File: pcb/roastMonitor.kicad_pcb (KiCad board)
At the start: 2 copper layers, 45 x 60 mm, 73 parts, among them J1 USB_C_Receptacle_USB2.0_16P, J2 Conn_01x02, J3 Conn_01x02, J4 Conn_01x04, J5 Conn_01x04, U1 REF3040, U2 USBLC6-2SC6, U3 OPA2333xxD, U4 CH32X033F8P6, U5 MCP9701A, U6 OPA2333xxD

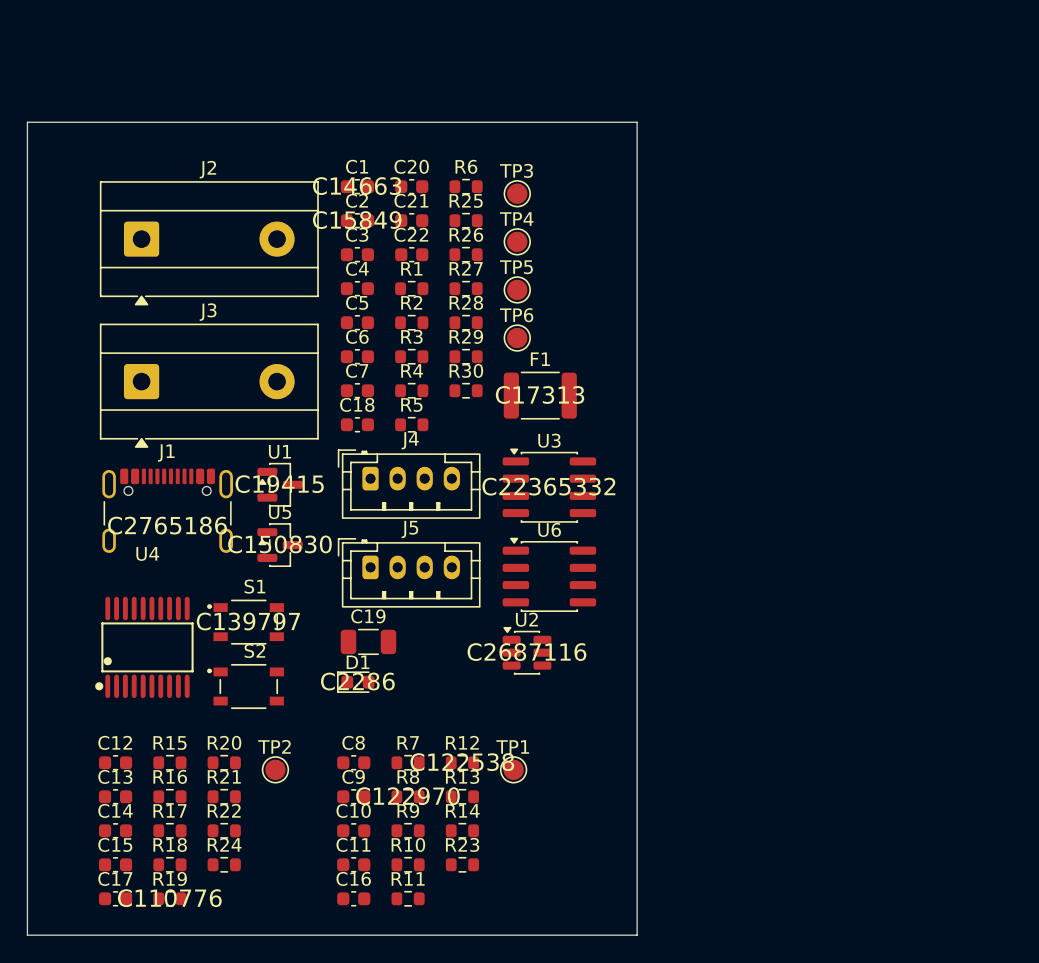
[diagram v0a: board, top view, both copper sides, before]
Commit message: Update PCB
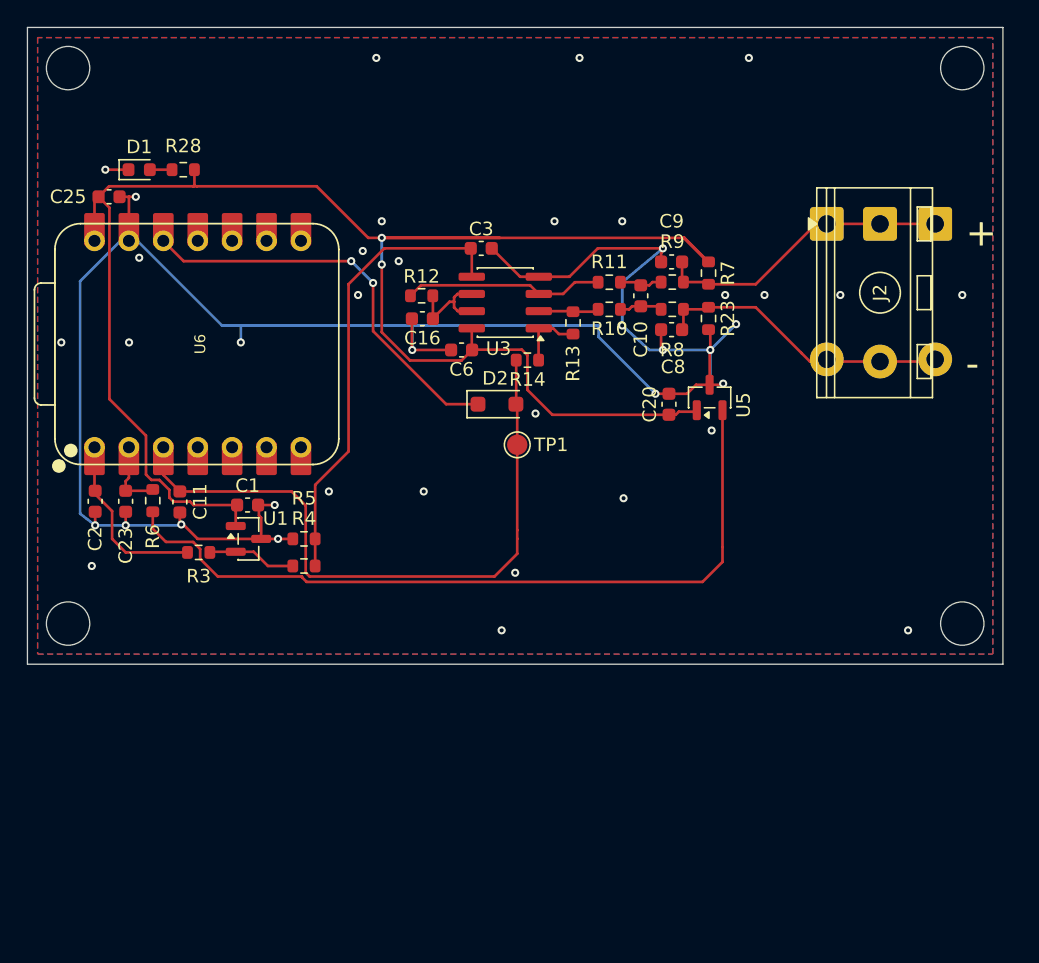
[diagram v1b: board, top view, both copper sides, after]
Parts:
- removed C12, C13, C14, C17, C18, C21, C22, C4, C5, C7: 100n, Capacitor_SMD:C_0603_1608Metric
- removed C15: 1u, Capacitor_SMD:C_0603_1608Metric
- removed C19: 4.7u, Capacitor_SMD:C_1206_3216Metric
- removed F1: Polyfuse, Fuse:Fuse_1812_4532Metric
- removed J1: USB_C_Receptacle_USB2.0_16P, Connector_USB:USB_C_Receptacle_GCT_USB4105-xx-A_16P_TopMnt_Horizontal
- removed J3: Conn_01x02, TerminalBlock_MetzConnect:TerminalBlock_MetzConnect_Type067_RT01902HDWC_1x02_P10.00mm_Horizontal
- removed J4, J5: Conn_01x04, Connector_JST:JST_PH_B4B-PH-K_1x04_P2.00mm_Vertical
- removed R1, R2: 5.1k, Resistor_SMD:R_0603_1608Metric
- removed R15: 10M, Resistor_SMD:R_0603_1608Metric
- removed R16, R17: 100±0.1%, Resistor_SMD:R_0603_1608Metric
- removed R18, R19: 1k±0.1%, Resistor_SMD:R_0603_1608Metric
- removed R20, R21: 100k±0.1%, Resistor_SMD:R_0603_1608Metric
- removed R22: 1k, Resistor_SMD:R_0603_1608Metric
- removed R24: 0, Resistor_SMD:R_0603_1608Metric
- removed R25, R26, R29, R30: 22, Resistor_SMD:R_0603_1608Metric
- removed R27: 10k, Resistor_SMD:R_0603_1608Metric
- removed S1, S2: SKRPACE010, private:SW_SKRPACE010
- removed TP2, TP3, TP4, TP5, TP6: TestPoint, TestPoint:TestPoint_Pad_D1.5mm
- removed U2: USBLC6-2SC6, Package_TO_SOT_SMD:SOT-23-6
- removed U4: CH32X033F8P6, private:TSSOP-20_L6.5-W4.4-P0.65-LS6.4-BL
- added ?: , , F.Cu at (197.0, 87.5)
- added ?: , , F.Cu at (189.0, 87.5)
- added ?: , , F.Cu at (189.0, 77.5)
- added ?: , , F.Cu at (197.0, 77.5)
- added C23: 1u, Capacitor_SMD:C_0603_1608Metric, F.Cu at (137.2, 98.0)
- added C25: 100n, Capacitor_SMD:C_0603_1608Metric, F.Cu at (136.0, 75.5)
- added D2: D, Diode_SMD:D_SOD-123F, F.Cu at (164.7, 90.8)
- added H1: MountingHole, MountingHole:MountingHole_3.2mm_M3, F.Cu at (133.0, 107.0)
- added H2: MountingHole, MountingHole:MountingHole_3.2mm_M3, F.Cu at (199.0, 107.0)
- added H3: MountingHole, MountingHole:MountingHole_3.2mm_M3, F.Cu at (199.0, 66.0)
- added H4: MountingHole, MountingHole:MountingHole_3.2mm_M3, F.Cu at (133.0, 66.0)
- J2: footprint TerminalBlock_MetzConnect:TerminalBlock_MetzConnect_Type067_RT01902HDWC_1x02_P10.00mm_Horizontal -> TerminalBlock_RND:TerminalBlock_RND_205-00241_1x02_P10.16mm_Horizontal
- R4, R5: value 100k -> 100k±0.1%
- U6: value OPA2333xxD -> XIAO-ESP32-C3-DIP; footprint Package_SO:SOIC-8_3.9x4.9mm_P1.27mm -> private:XIAO-ESP32-C3-DIP
- moved J2 54.5 mm to (192.9, 77.5), turned to -90 degrees
- moved R11 47.9 mm to (172.9, 81.8), turned to 180 degrees
- moved C9 45.9 mm to (177.5, 80.3), turned to 180 degrees
- moved R9 44.9 mm to (177.6, 81.8), turned to 180 degrees
- moved C10 44.8 mm to (175.3, 82.8), turned to 90 degrees
- moved R23 44.2 mm to (180.3, 84.5), turned to -90 degrees
- moved R10 43.6 mm to (172.9, 83.8), turned to 180 degrees
- moved C16 43.1 mm to (159.2, 84.5), turned to 180 degrees
- moved R7 42.4 mm to (180.3, 81.1), turned to -90 degrees
- moved D1 41.1 mm to (138.2, 73.5)
- moved R8 40.9 mm to (177.6, 83.8), turned to 180 degrees
- moved C8 39.7 mm to (177.5, 85.3), turned to 180 degrees
- moved R13 35.9 mm to (170.3, 84.8), turned to -90 degrees
- moved R14 35.1 mm to (166.9, 87.6), turned to 180 degrees
- moved R12 34.6 mm to (159.1, 82.8)
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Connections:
- R6 pad 1: Net-(U4-PA5) -> Net-(U5-V_{OUT})
- R6 pad 2: Net-(U5-V_{OUT}) -> /Vtemp
- U6 pad 1: Net-(R21-Pad2) -> /Vref
- U6 pad 2: Net-(U6A--) -> /Vtemp
- U6 pad 3: Net-(U6A-+) -> /Vthermo1
- U6 pad 4: GND -> unconnected-(U6-GPIO5_A3_D3-Pad4)
- U6 pad 5: GND -> unconnected-(U6-GPIO6_D4_SDA-Pad5)
- U6 pad 6: Net-(U6B--) -> unconnected-(U6-GPIO7_D5_SCL-Pad6)
- U6 pad 7: Net-(U6B--) -> unconnected-(U6-GPIO21_D6_TX-Pad7)
- U6 pad 8: +5V -> unconnected-(U6-GPIO20_D7_RX-Pad8)_1
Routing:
- net GND: track 0.00 -> 151.9 mm, vias 0 -> 41
- net +5V: track 0.00 -> 132.2 mm, vias 0 -> 2
- net Net-(U5-V_{OUT}): track 0.00 -> 57.2 mm
- net /Vthermo1: track 0.00 -> 49.4 mm
- net Net-(U3B-+): track 0.00 -> 34.4 mm
- net Net-(D2-K): track 0.00 -> 30.3 mm, vias 0 -> 2
- net /amp/ThermoCouple+: track 0.00 -> 22.0 mm
- net /amp/ThermoCouple-: track 0.00 -> 21.9 mm
- net Net-(U3A-+): track 0.00 -> 14.8 mm
- net /Vref: track 0.00 -> 13.4 mm
- net /amp/Voffset: track 0.00 -> 7.58 mm
- net Net-(U1-OUT): track 0.00 -> 6.58 mm
- net /Vtemp: track 0.00 -> 5.14 mm
- net Net-(R13-Pad2): track 0.00 -> 5.05 mm
- net Net-(U3A--): track 0.00 -> 4.46 mm
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- added copper zone on B.Cu, net GND
- added copper zone on F.Cu, net GND
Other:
- board size 45 x 60 mm -> 72 x 47 mm
- board text added: "+ -"
